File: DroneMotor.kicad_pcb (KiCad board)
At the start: 2 copper layers, 184 x 184 mm, 49 parts, among them Q1 ISCH54N04NM7V, Q10 ISCH54N04NM7V, Q11 ISCH54N04NM7V, Q12 ISCH54N04NM7V, Q13 ISCH54N04NM7V, Q14 ISCH54N04NM7V, Q15 ISCH54N04NM7V, Q16 ISCH54N04NM7V, Q17 ISCH54N04NM7V, Q18 ISCH54N04NM7V, Q19 ISCH54N04NM7V, Q2 ISCH54N04NM7V, Q20 ISCH54N04NM7V, Q21 ISCH54N04NM7V, Q22 ISCH54N04NM7V, Q23 ISCH54N04NM7V, Q24 ISCH54N04NM7V, Q3 ISCH54N04NM7V, Q4 ISCH54N04NM7V, Q5 ISCH54N04NM7V, Q6 ISCH54N04NM7V, Q7 ISCH54N04NM7V, Q8 ISCH54N04NM7V, Q9 ISCH54N04NM7V, U1 MKV58F1M0VLQ22, U10 UCC27211DRMR, U11 UCC27211DRMR, U12 UCC27211DRMR, U13 UCC27211DRMR, U2 UCC27211DRMR, U3 UCC27211DRMR, U4 UCC27211DRMR, U5 UCC27211DRMR, U6 UCC27211DRMR, U7 UCC27211DRMR, U8 UCC27211DRMR, U9 UCC27211DRMR

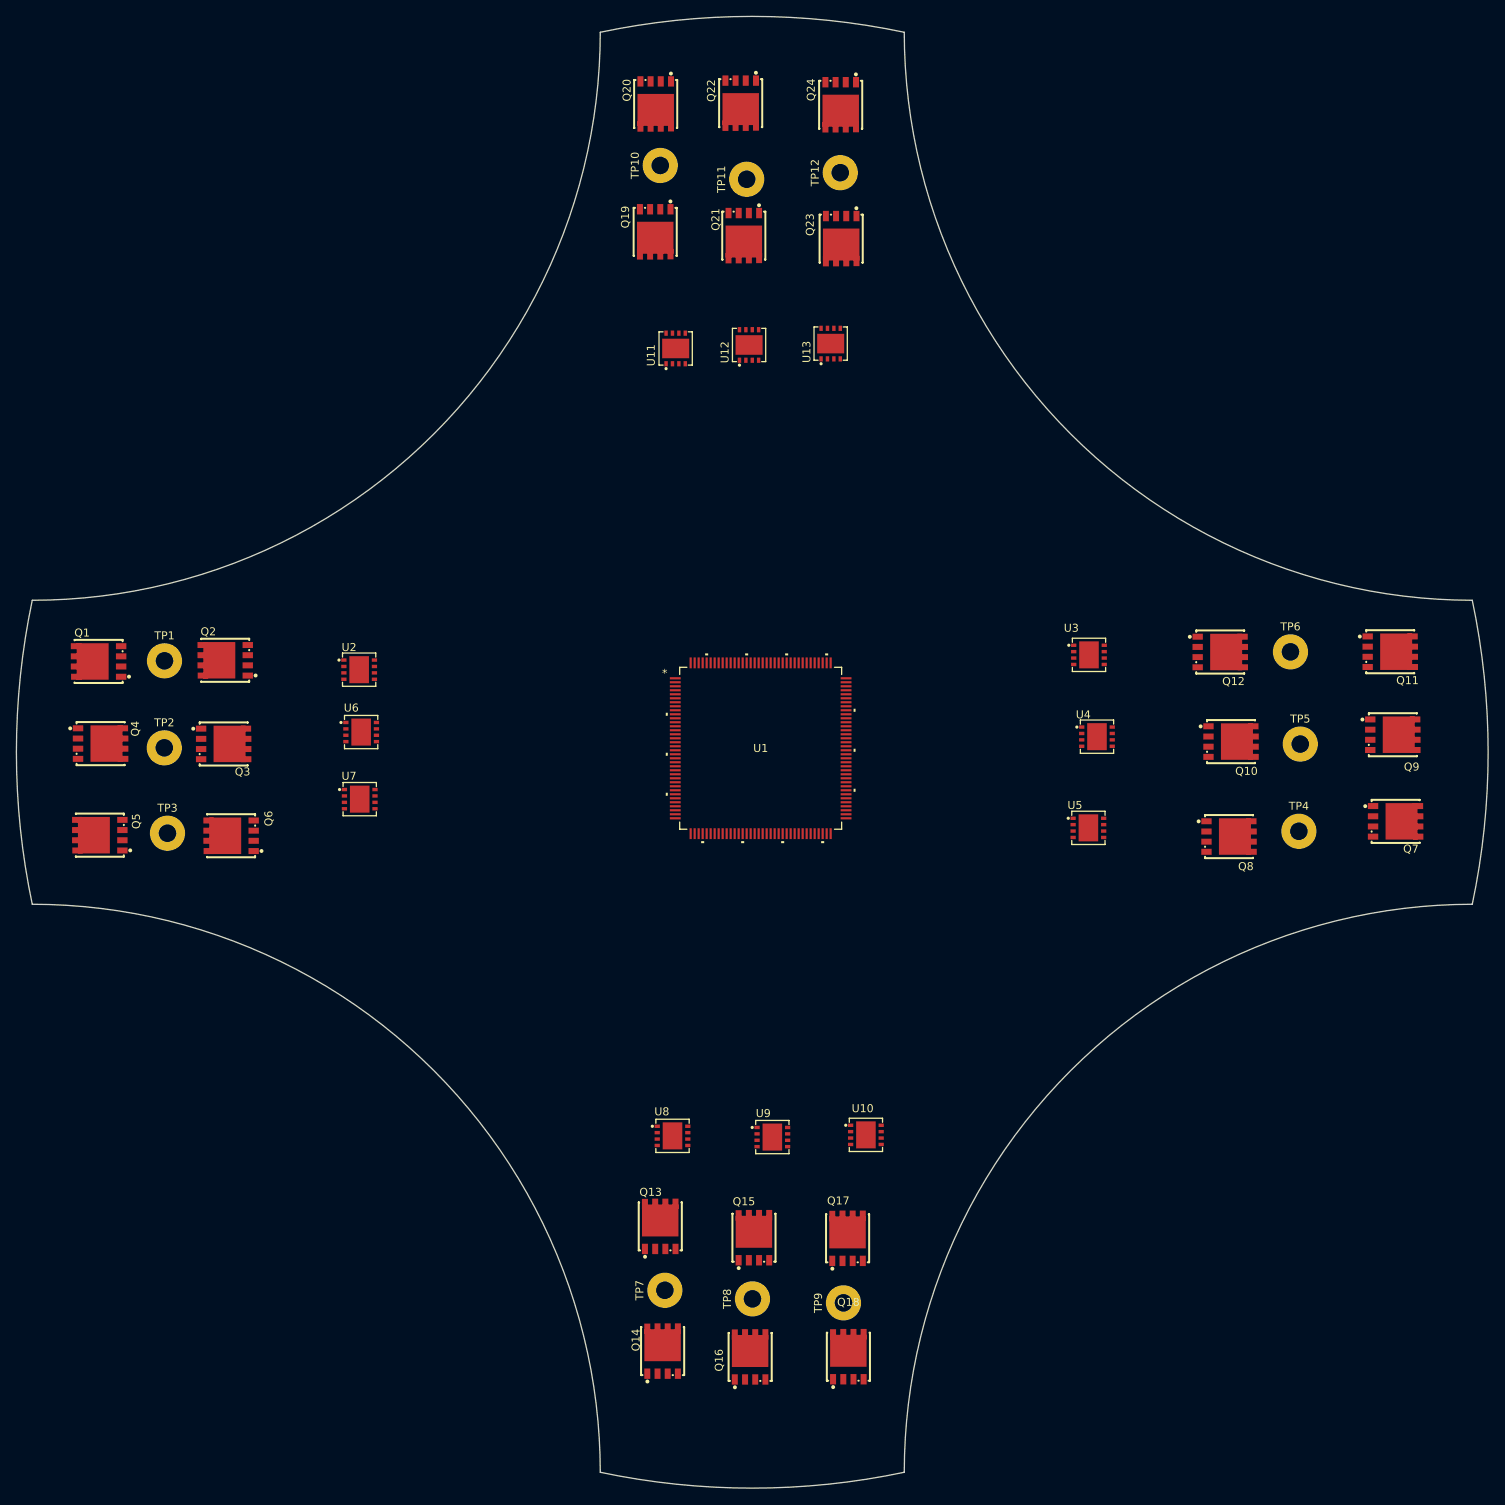
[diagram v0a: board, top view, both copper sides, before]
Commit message: add ti version
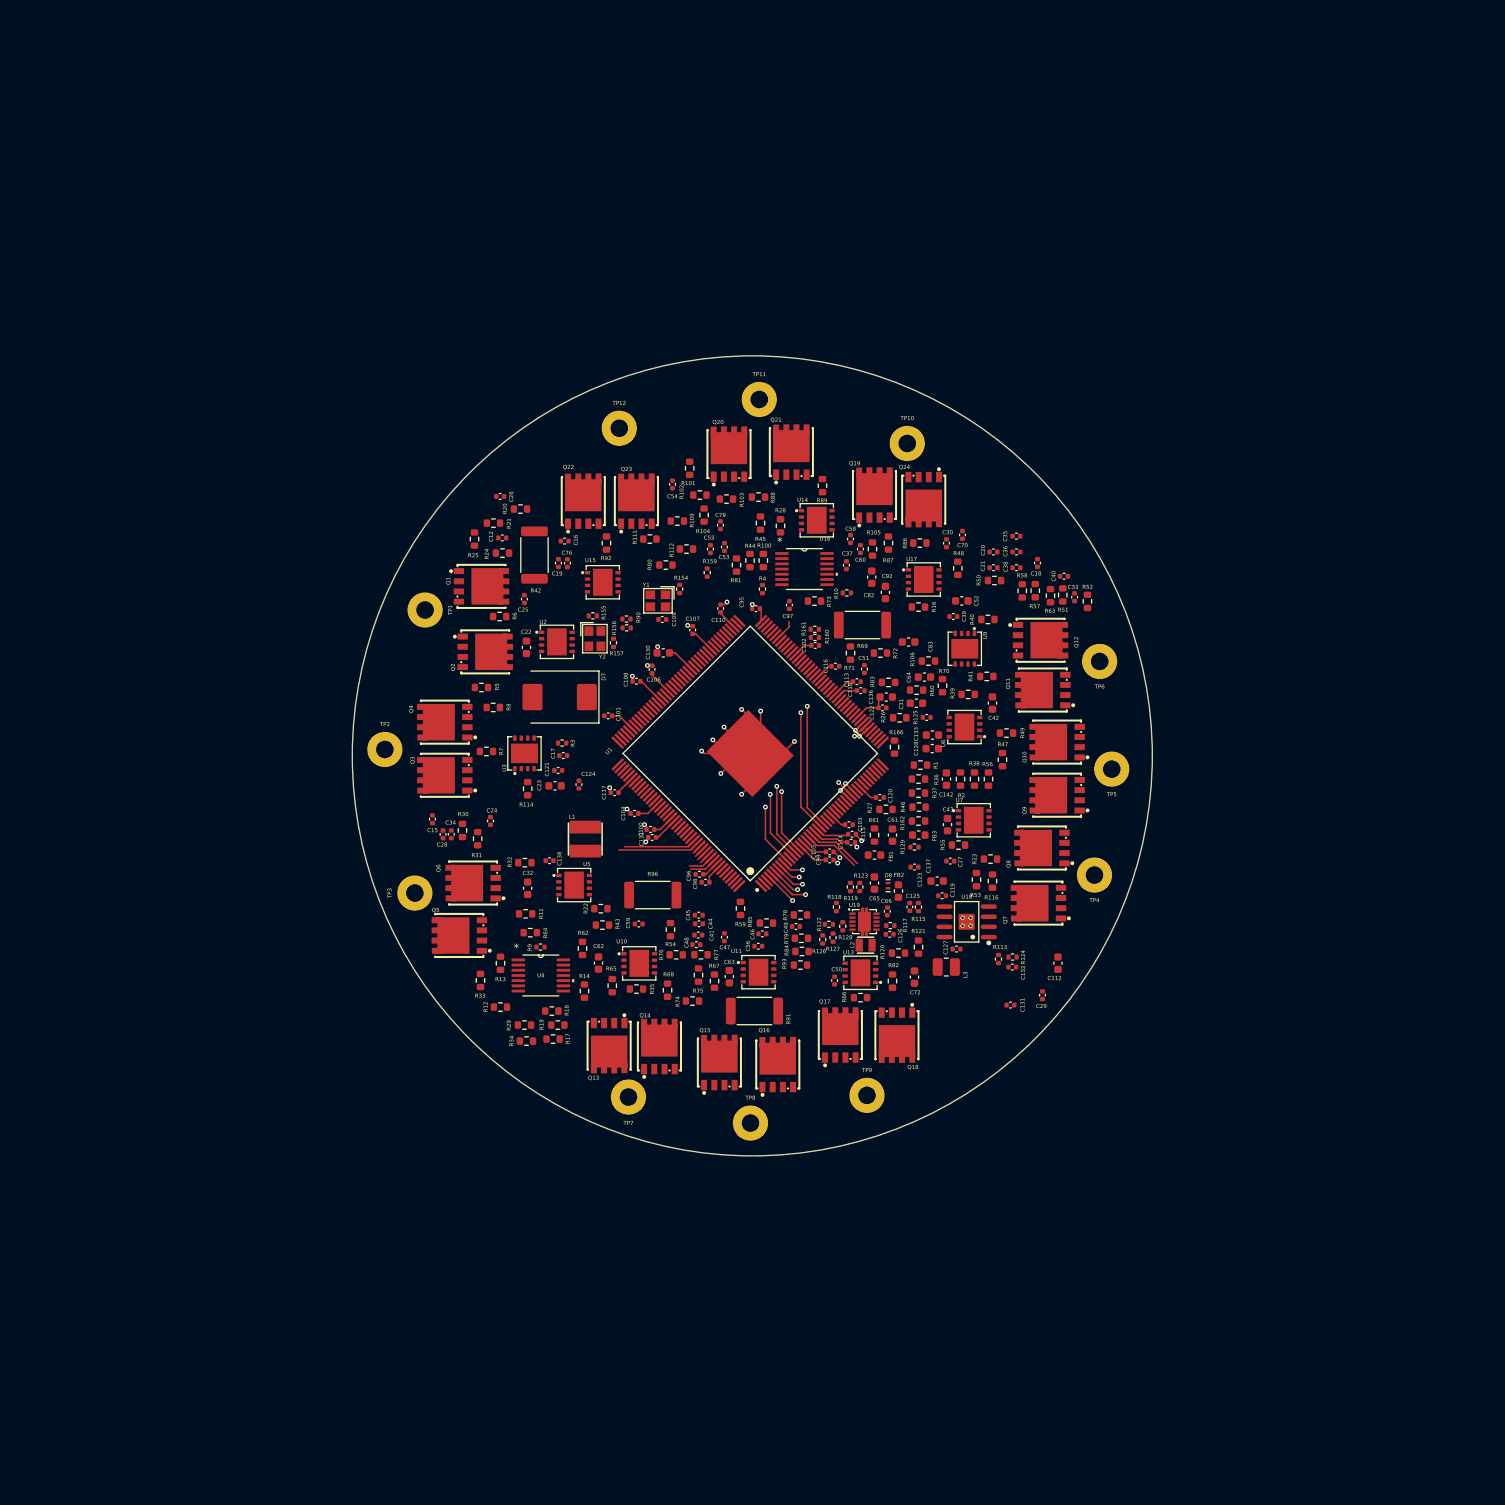
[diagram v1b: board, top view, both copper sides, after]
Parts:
- removed U12, U8: UCC27211DRMR, footprints:VSON-8_L4.0-W4.0-P0.80-TL-EP
- added C100: 0.1uF, Capacitor_SMD:C_0402_1005Metric, F.Cu at (202.0, 150.8)
- added C101: 0.1uF, Capacitor_SMD:C_0402_1005Metric, F.Cu at (196.7, 136.6)
- added C102: 0.1uF, Capacitor_SMD:C_0402_1005Metric, F.Cu at (222.6, 127.8)
- added C103: 0.1uF, Capacitor_SMD:C_0402_1005Metric, F.Cu at (226.8, 150.2)
- added C104: 0.1uF, Capacitor_SMD:C_0402_1005Metric, F.Cu at (200.0, 148.8)
- added C105: 0.1uF, Capacitor_SMD:C_0402_1005Metric, F.Cu at (224.4, 153.6)
- added C106: 0.1uF, Capacitor_SMD:C_0402_1005Metric, F.Cu at (202.2, 130.8)
- added C107: 0.1uF, Capacitor_SMD:C_0402_1005Metric, F.Cu at (207.3, 125.9)
- added C108: 0.1uF, Capacitor_SMD:C_0402_1005Metric, F.Cu at (200.2, 132.3)
- added C109: 0.1uF, Capacitor_SMD:C_0402_1005Metric, F.Cu at (203.5, 124.5)
- added C110: 0.1uF, Capacitor_SMD:C_0402_1005Metric, F.Cu at (210.8, 123.2)
- added C111: 0.1uF, Capacitor_SMD:C_0402_1005Metric, F.Cu at (202.2, 151.8)
- added C112: 3.3uF, Capacitor_SMD:C_0603_1608Metric, F.Cu at (252.9, 167.5)
- added C113: 0.1uF, Capacitor_SMD:C_0402_1005Metric, F.Cu at (227.8, 132.3)
- added C114: 0.1uF, Capacitor_SMD:C_0402_1005Metric, F.Cu at (227.1, 152.4)
- added C115: 0.1uF, Capacitor_SMD:C_0402_1005Metric, F.Cu at (227.2, 151.4)
- added C116: 0.1uF, Capacitor_SMD:C_0402_1005Metric, F.Cu at (225.1, 130.4)
- added C117: 0.1uF, Capacitor_SMD:C_0402_1005Metric, F.Cu at (197.5, 146.2)
- added C118: 0.1uF, Capacitor_SMD:C_0402_1005Metric, F.Cu at (228.3, 133.4)
- added C119: 0.1uF, Capacitor_SMD:C_0402_1005Metric, F.Cu at (238.5, 159.1)
- added C12: 2.2uF, Capacitor_SMD:C_0402_1005Metric, F.Cu at (183.5, 114.4)
- added C120: 0.1uF, Capacitor_SMD:C_0402_1005Metric, F.Cu at (230.7, 146.8)
- added C121: 1800pF, Capacitor_SMD:C_0402_1005Metric, F.Cu at (190.5, 143.4)
- added C122: 0.1uF, Capacitor_SMD:C_0402_1005Metric, F.Cu at (231.0, 135.6)
- added C123: 22uF, Capacitor_SMD:C_0603_1608Metric, F.Cu at (237.8, 157.2)
- added C124: 56pF, Capacitor_SMD:C_0402_1005Metric, F.Cu at (193.1, 145.2)
- added C125: 0.1uF, Capacitor_SMD:C_0402_1005Metric, F.Cu at (234.4, 160.5)
- added C126: 0.1uF, Capacitor_SMD:C_0402_1005Metric, F.Cu at (231.9, 163.9)
- added C127: 0.1uF, Capacitor_SMD:C_0402_1005Metric, F.Cu at (240.2, 165.8)
- added C128: 2.2uF, Capacitor_SMD:C_0603_1608Metric, F.Cu at (237.2, 140.7)
- added C130: 2.2uF, Capacitor_SMD:C_0603_1608Metric, F.Cu at (203.6, 128.7)
- added C131: 10uF, Capacitor_SMD:C_0402_1005Metric, F.Cu at (247.0, 172.8)
- added C132: 33pF, Capacitor_SMD:C_0402_1005Metric, F.Cu at (247.2, 168.0)
- added C133: 2.2uF, Capacitor_SMD:C_0603_1608Metric, F.Cu at (237.2, 139.0)
- added C136: 2.2uF, Capacitor_SMD:C_0603_1608Metric, F.Cu at (231.5, 134.2)
- added C137: 22uF, Capacitor_SMD:C_0402_1005Metric, F.Cu at (235.0, 155.5)
- added C138: 2.2uF, Capacitor_SMD:C_0402_1005Metric, F.Cu at (189.4, 154.7)
- added C142: 22uF, Capacitor_SMD:C_0603_1608Metric, F.Cu at (239.0, 144.5)
- added C15: 2.2uF, Capacitor_SMD:C_0402_1005Metric, F.Cu at (174.8, 149.5)
- added C16: 2.2uF, Capacitor_SMD:C_0402_1005Metric, F.Cu at (191.3, 114.8)
- added C17: 0.1uF, Capacitor_SMD:C_0402_1005Metric, F.Cu at (191.1, 141.6)
- added C18: 0.1uF, Capacitor_SMD:C_0402_1005Metric, F.Cu at (250.4, 117.5)
- added C19: 2.2uF, Capacitor_SMD:C_0402_1005Metric, F.Cu at (190.5, 117.5)
- added C20: 0.1uF, Capacitor_SMD:C_0402_1005Metric, F.Cu at (244.9, 116.1)
- added C21: 0.1uF, Capacitor_SMD:C_0402_1005Metric, F.Cu at (244.9, 118.1)
- added C22: 0.1uF, Capacitor_SMD:C_0603_1608Metric, F.Cu at (186.5, 128.0)
- added C23: 0.1uF, Capacitor_SMD:C_0603_1608Metric, F.Cu at (190.1, 145.3)
- added C24: 2.2uF, Capacitor_SMD:C_0402_1005Metric, F.Cu at (182.0, 149.7)
- added C25: 2.2uF, Capacitor_SMD:C_0402_1005Metric, F.Cu at (186.2, 122.0)
- added C26: 0.1uF, Capacitor_SMD:C_0402_1005Metric, F.Cu at (183.2, 109.2)
- added C27: 0.1uF, Capacitor_SMD:C_0402_1005Metric, F.Cu at (239.5, 154.8)
- added C28: 0.1uF, Capacitor_SMD:C_0402_1005Metric, F.Cu at (176.1, 151.4)
- added C29: 0.1uF, Capacitor_SMD:C_0402_1005Metric, F.Cu at (251.0, 171.5)
- added C30: 2.2uF, Capacitor_SMD:C_0402_1005Metric, F.Cu at (239.0, 115.0)
- added C31: 22uF, Capacitor_SMD:C_0603_1608Metric, F.Cu at (235.2, 135.0)
- added C32: 0.1uF, Capacitor_SMD:C_0603_1608Metric, F.Cu at (186.7, 158.2)
- added C33: 0.1uF, Capacitor_SMD:C_0402_1005Metric, F.Cu at (255.0, 121.8)
- added C34: 0.1uF, Capacitor_SMD:C_0402_1005Metric, F.Cu at (177.1, 151.4)
- added C35: 2.2uF, Capacitor_SMD:C_0402_1005Metric, F.Cu at (247.7, 114.1)
- added C36: 2.2uF, Capacitor_SMD:C_0402_1005Metric, F.Cu at (247.7, 116.1)
- added C37: 0.1uF, Capacitor_SMD:C_0402_1005Metric, F.Cu at (226.5, 117.8)
- added C38: 2.2uF, Capacitor_SMD:C_0402_1005Metric, F.Cu at (247.7, 118.1)
- added C39: 2.2uF, Capacitor_SMD:C_0402_1005Metric, F.Cu at (239.9, 124.2)
- added C40: 2.2uF, Capacitor_SMD:C_0402_1005Metric, F.Cu at (253.7, 119.2)
- added C41: 2.2uF, Capacitor_SMD:C_0402_1005Metric, F.Cu at (208.0, 164.0)
- added C42: 0.1uF, Capacitor_SMD:C_0603_1608Metric, F.Cu at (244.8, 135.0)
- added C43: 0.1uF, Capacitor_SMD:C_0603_1608Metric, F.Cu at (239.1, 150.2)
- added C44: 2.2uF, Capacitor_SMD:C_0402_1005Metric, F.Cu at (208.1, 162.6)
- added C45: 2.2uF, Capacitor_SMD:C_0402_1005Metric, F.Cu at (208.0, 161.5)
- added C46: 0.1uF, Capacitor_SMD:C_0402_1005Metric, F.Cu at (216.0, 163.8)
- added C47: 0.1uF, Capacitor_SMD:C_0402_1005Metric, F.Cu at (211.2, 164.3)
- added C48: 0.1uF, Capacitor_SMD:C_0402_1005Metric, F.Cu at (207.7, 165.2)
- added C49: 0.1uF, Capacitor_SMD:C_0402_1005Metric, F.Cu at (220.2, 162.9)
- added C50: 2.2uF, Capacitor_SMD:C_0402_1005Metric, F.Cu at (225.0, 169.7)
- added C51: 0.1uF, Capacitor_SMD:C_0402_1005Metric, F.Cu at (228.8, 130.8)
- added C52: 0.1uF, Capacitor_SMD:C_0603_1608Metric, F.Cu at (240.9, 122.2)
- added C53: 0.1uF, Capacitor_SMD:C_0402_1005Metric, F.Cu at (211.2, 115.5)
- added C54: 0.1uF, Capacitor_SMD:C_0402_1005Metric, F.Cu at (204.8, 107.7)
- added C55: 0.1uF, Capacitor_SMD:C_0402_1005Metric, F.Cu at (209.5, 115.8)
- added C56: 2.2uF, Capacitor_SMD:C_0402_1005Metric, F.Cu at (215.5, 165.4)
- added C58: 2.2uF, Capacitor_SMD:C_0402_1005Metric, F.Cu at (227.0, 114.5)
- added C59: 2.2uF, Capacitor_SMD:C_0402_1005Metric, F.Cu at (200.5, 162.6)
- added C60: 2.2uF, Capacitor_SMD:C_0402_1005Metric, F.Cu at (228.2, 115.8)
- added C61: 22uF, Capacitor_SMD:C_0603_1608Metric, F.Cu at (232.2, 151.5)
- added C62: 0.1uF, Capacitor_SMD:C_0603_1608Metric, F.Cu at (195.5, 167.5)
- added C63: 0.1uF, Capacitor_SMD:C_0603_1608Metric, F.Cu at (211.9, 169.2)
- added C64: 22uF, Capacitor_SMD:C_0603_1608Metric, F.Cu at (236.2, 131.8)
- added C65: 22uF, Capacitor_SMD:C_0603_1608Metric, F.Cu at (230.0, 157.5)
- added C66: 10uF, Capacitor_SMD:C_0402_1005Metric, F.Cu at (231.6, 161.0)
- added C70: 2.2uF, Capacitor_SMD:C_0402_1005Metric, F.Cu at (241.0, 114.0)
- added C72: 0.1uF, Capacitor_SMD:C_0603_1608Metric, F.Cu at (235.0, 169.2)
- added C76: 2.2uF, Capacitor_SMD:C_0402_1005Metric, F.Cu at (191.6, 117.5)
- added C79: 2.2uF, Capacitor_SMD:C_0402_1005Metric, F.Cu at (210.8, 112.8)
- added C82: 0.1uF, Capacitor_SMD:C_0603_1608Metric, F.Cu at (229.7, 119.3)
- added C83: 0.1uF, Capacitor_SMD:C_0603_1608Metric, F.Cu at (234.3, 127.4)
- added C92: 0.1uF, Capacitor_SMD:C_0603_1608Metric, F.Cu at (231.4, 121.2)
- added C95: 0.1uF, Capacitor_SMD:C_0402_1005Metric, F.Cu at (215.2, 123.2)
- added C96: 0.1uF, Capacitor_SMD:C_0402_1005Metric, F.Cu at (208.1, 156.4)
- added C97: 0.1uF, Capacitor_SMD:C_0402_1005Metric, F.Cu at (219.4, 122.7)
- added C98: 0.1uF, Capacitor_SMD:C_0402_1005Metric, F.Cu at (208.9, 157.4)
- added C99: 0.1uF, Capacitor_SMD:C_0402_1005Metric, F.Cu at (224.4, 154.6)
- added D7: SS510-SMC, Diode_SMD:D_SMC, F.Cu at (190.7, 134.2)
- added D8: CFSH05-20L, footprints:SOD-882_L1.0-W0.6-BI, F.Cu at (231.7, 157.8)
- added FB1: 60, Inductor_SMD:L_0603_1608Metric, F.Cu at (230.0, 154.0)
- added FB2: 220, Inductor_SMD:L_0603_1608Metric, F.Cu at (233.0, 158.5)
- added FB3: 60, Inductor_SMD:L_0603_1608Metric, F.Cu at (235.5, 151.5)
- added L1: 33uH, footprints:IND-SMD_L4.0-W4.0_FNR40XXS, F.Cu at (193.8, 152.0)
- added L2: VLS201612HBX-2R2M-1, footprints:IND-SMD_L2.0-W1.6_VLS201610ET, F.Cu at (228.9, 165.3)
- added L3: 3.3uH, Inductor_SMD:L_1008_2520Metric, F.Cu at (239.0, 168.0)
- added R1: 56.0, Resistor_SMD:R_0603_1608Metric, F.Cu at (235.8, 142.8)
- added R10: 330, Resistor_SMD:R_0402_1005Metric, F.Cu at (226.6, 121.2)
- added R100: 33K, Resistor_SMD:R_0603_1608Metric, F.Cu at (216.1, 117.2)
- added R101: 68K, Resistor_SMD:R_0603_1608Metric, F.Cu at (206.9, 105.7)
- added R102: 18K, Resistor_SMD:R_0603_1608Metric, F.Cu at (208.2, 109.0)
- added R103: 68K, Resistor_SMD:R_0603_1608Metric, F.Cu at (211.5, 109.5)
- added R104: 18K, Resistor_SMD:R_0603_1608Metric, F.Cu at (208.7, 111.5)
- added R105: 68K, Resistor_SMD:R_0603_1608Metric, F.Cu at (229.8, 115.8)
- added R106: 18K, Resistor_SMD:R_0603_1608Metric, F.Cu at (236.8, 129.8)
- added R109: 10, Resistor_SMD:R_0603_1608Metric, F.Cu at (205.4, 112.2)
- added R11: 10, Resistor_SMD:R_0603_1608Metric, F.Cu at (186.4, 161.3)
- added R111: 68K, Resistor_SMD:R_0603_1608Metric, F.Cu at (201.9, 114.5)
- added R112: 18K, Resistor_SMD:R_0603_1608Metric, F.Cu at (206.5, 115.8)
- added R113: 0, Resistor_SMD:R_0402_1005Metric, F.Cu at (245.5, 167.0)
- added R114: 32.4k, Resistor_SMD:R_0603_1608Metric, F.Cu at (186.7, 145.7)
- added R115: 22K, Resistor_SMD:R_0402_1005Metric, F.Cu at (235.5, 160.5)
- added R116: 178K, Resistor_SMD:R_0603_1608Metric, F.Cu at (244.8, 157.2)
- added R117: 0, Resistor_SMD:R_0402_1005Metric, F.Cu at (232.0, 162.8)
- added R118: 10K, Resistor_SMD:R_0402_1005Metric, F.Cu at (225.2, 160.5)
- added R119: 100K, Resistor_SMD:R_0402_1005Metric, F.Cu at (227.0, 158.0)
- added R12: 33K, Resistor_SMD:R_0603_1608Metric, F.Cu at (183.2, 173.0)
- added R120: 118K, Resistor_SMD:R_0603_1608Metric, F.Cu at (233.0, 166.2)
- added R121: 8.45K, Resistor_SMD:R_0603_1608Metric, F.Cu at (235.5, 165.5)
- added R122: 0, Resistor_SMD:R_0402_1005Metric, F.Cu at (224.3, 162.7)
- added R123: 56, Resistor_SMD:R_0402_1005Metric, F.Cu at (228.2, 158.0)
- added R124: 205K, Resistor_SMD:R_0402_1005Metric, F.Cu at (247.3, 166.8)
- added R125: 200K, Capacitor_SMD:C_0402_1005Metric, F.Cu at (236.5, 136.8)
- added R126: 340K, Resistor_SMD:R_0402_1005Metric, F.Cu at (223.5, 164.6)
- added R127: 2.00K, Resistor_SMD:R_0402_1005Metric, F.Cu at (224.8, 164.3)
- added R128: 75K, Resistor_SMD:R_0402_1005Metric, F.Cu at (226.0, 162.9)
- added R129: 680, Resistor_SMD:R_0402_1005Metric, F.Cu at (235.0, 153.0)
- added R13: 33K, Resistor_SMD:R_0603_1608Metric, F.Cu at (183.2, 167.5)
- added R14: 33K, Resistor_SMD:R_0603_1608Metric, F.Cu at (193.8, 171.0)
- added R154: 0, Resistor_SMD:R_0402_1005Metric, F.Cu at (205.7, 120.8)
- added R155: 0, Resistor_SMD:R_0402_1005Metric, F.Cu at (194.8, 124.1)
- added R156: 0, Resistor_SMD:R_0402_1005Metric, F.Cu at (199.0, 125.6)
- added R157: 0, Resistor_SMD:R_0402_1005Metric, F.Cu at (197.4, 127.5)
- added R159: 10K, Resistor_SMD:R_0402_1005Metric, F.Cu at (209.1, 118.7)
- added R16: 1K, Resistor_SMD:R_0603_1608Metric, F.Cu at (235.5, 123.0)
- added R160: 39, Resistor_SMD:R_0402_1005Metric, F.Cu at (222.6, 126.8)
- added R161: 2.2K, Resistor_SMD:R_0402_1005Metric, F.Cu at (222.5, 125.8)
- added R162: 0.1, Resistor_SMD:R_0603_1608Metric, F.Cu at (235.5, 149.8)
- added R166: 56.0, Resistor_SMD:R_0603_1608Metric, F.Cu at (232.5, 140.5)
- added R17: 1K, Resistor_SMD:R_0603_1608Metric, F.Cu at (189.8, 177.0)
- added R18: 33K, Resistor_SMD:R_0603_1608Metric, F.Cu at (189.7, 173.5)
- added R19: 33K, Resistor_SMD:R_0603_1608Metric, F.Cu at (190.4, 175.2)
- added R2: 56.0, Resistor_SMD:R_0603_1608Metric, F.Cu at (240.8, 144.5)
- added R20: 68K, Resistor_SMD:R_0603_1608Metric, F.Cu at (185.8, 110.8)
- added R21: 18K, Resistor_SMD:R_0603_1608Metric, F.Cu at (182.4, 112.5)
- added R22: 68K, Resistor_SMD:R_0603_1608Metric, F.Cu at (195.8, 160.7)
- added R23: 18K, Resistor_SMD:R_0603_1608Metric, F.Cu at (244.5, 154.5)
- added R24: 68K, Resistor_SMD:R_0603_1608Metric, F.Cu at (183.5, 116.2)
- added R25: 18K, Resistor_SMD:R_0603_1608Metric, F.Cu at (180.0, 114.5)
- added R26: 0.1, Resistor_SMD:R_0603_1608Metric, F.Cu at (233.2, 136.8)
- added R27: 0.1, Resistor_SMD:R_0603_1608Metric, F.Cu at (231.4, 148.3)
- added R28: 33K, Resistor_SMD:R_0603_1608Metric, F.Cu at (218.2, 112.8)
- added R29: 33K, Resistor_SMD:R_0603_1608Metric, F.Cu at (186.2, 175.2)
- added R3: 330, Resistor_SMD:R_0402_1005Metric, F.Cu at (191.0, 140.0)
- added R30: 68K, Resistor_SMD:R_0603_1608Metric, F.Cu at (178.5, 150.9)
- added R31: 18K, Resistor_SMD:R_0603_1608Metric, F.Cu at (180.4, 151.9)
- added R32: 10, Resistor_SMD:R_0603_1608Metric, F.Cu at (186.3, 154.9)
- added R33: 1K, Resistor_SMD:R_0603_1608Metric, F.Cu at (180.8, 169.7)
- added R34: 1K, Resistor_SMD:R_0603_1608Metric, F.Cu at (186.5, 177.2)
- added R35: 1K, Resistor_SMD:R_0603_1608Metric, F.Cu at (200.2, 170.8)
- added R36: 56.0, Resistor_SMD:R_0603_1608Metric, F.Cu at (235.5, 144.5)
- added R37: 56.0, Resistor_SMD:R_0603_1608Metric, F.Cu at (235.5, 146.2)
- added R38: 10, Resistor_SMD:R_0603_1608Metric, F.Cu at (242.5, 144.5)
- added R39: 10, Resistor_SMD:R_0603_1608Metric, F.Cu at (241.7, 133.9)
- added R4: 330, Resistor_SMD:R_0402_1005Metric, F.Cu at (216.0, 120.8)
- added R40: 10, Resistor_SMD:R_0603_1608Metric, F.Cu at (244.2, 124.5)
- added R41: 10, Resistor_SMD:R_0603_1608Metric, F.Cu at (244.0, 131.7)
- added R42: 0.002, Resistor_SMD:R_2512_6332Metric, F.Cu at (187.5, 116.5)
- added R43: 1K, Resistor_SMD:R_0603_1608Metric, F.Cu at (196.0, 162.8)
- added R44: 1K, Resistor_SMD:R_0603_1608Metric, F.Cu at (214.4, 117.2)
- added R45: 1K, Resistor_SMD:R_0603_1608Metric, F.Cu at (215.8, 112.5)
- added R46: 56.0, Resistor_SMD:R_0603_1608Metric, F.Cu at (235.6, 148.0)
- added R47: 68K, Resistor_SMD:R_0603_1608Metric, F.Cu at (246.0, 142.1)
- added R48: 18K, Resistor_SMD:R_0603_1608Metric, F.Cu at (240.4, 118.2)
- added R49: 68K, Resistor_SMD:R_0603_1608Metric, F.Cu at (246.5, 138.8)
- added R5: 10, Resistor_SMD:R_0603_1608Metric, F.Cu at (180.9, 133.1)
- added R50: 18K, Resistor_SMD:R_0603_1608Metric, F.Cu at (245.0, 119.7)
- added R51: 68K, Resistor_SMD:R_0603_1608Metric, F.Cu at (253.5, 121.5)
- added R52: 18K, Resistor_SMD:R_0603_1608Metric, F.Cu at (256.6, 122.3)
- added R53: 56.0, Resistor_SMD:R_0603_1608Metric, F.Cu at (242.8, 157.1)
- added R54: 56.0, Resistor_SMD:R_0603_1608Metric, F.Cu at (204.5, 163.3)
- added R55: 10, Resistor_SMD:R_0603_1608Metric, F.Cu at (240.5, 152.8)
- added R56: 10, Resistor_SMD:R_0603_1608Metric, F.Cu at (244.2, 144.5)
- added R57: 68K, Resistor_SMD:R_0603_1608Metric, F.Cu at (250.1, 121.0)
- added R58: 18K, Resistor_SMD:R_0603_1608Metric, F.Cu at (248.5, 121.0)
- added R59: 56.0, Resistor_SMD:R_0603_1608Metric, F.Cu at (213.2, 160.7)
- added R6: 10, Resistor_SMD:R_0603_1608Metric, F.Cu at (183.1, 124.2)
- added R60: 56.0, Resistor_SMD:R_0603_1608Metric, F.Cu at (235.3, 133.4)
- added R61: 56.0, Resistor_SMD:R_0603_1608Metric, F.Cu at (230.0, 151.5)
- added R62: 56.0, Resistor_SMD:R_0603_1608Metric, F.Cu at (193.5, 165.7)
- added R63: 56.0, Resistor_SMD:R_0603_1608Metric, F.Cu at (252.0, 121.6)
- added R64: 56.0, Resistor_SMD:R_0603_1608Metric, F.Cu at (187.0, 163.7)
- added R65: 10, Resistor_SMD:R_0603_1608Metric, F.Cu at (197.2, 170.3)
- added R66: 10, Resistor_SMD:R_0603_1608Metric, F.Cu at (228.2, 171.8)
- added R67: 10, Resistor_SMD:R_0603_1608Metric, F.Cu at (210.0, 169.8)
- added R68: 10, Resistor_SMD:R_0603_1608Metric, F.Cu at (204.1, 170.9)
- added R69: 0.002, Resistor_SMD:R_2512_6332Metric, F.Cu at (228.5, 125.2)
- added R7: 10, Resistor_SMD:R_0603_1608Metric, F.Cu at (181.5, 141.1)
- added R70: 56.0, Resistor_SMD:R_0603_1608Metric, F.Cu at (238.5, 132.8)
- added R71: 56.0, Resistor_SMD:R_0603_1608Metric, F.Cu at (227.0, 128.8)
- added R72: 56.0, Resistor_SMD:R_0603_1608Metric, F.Cu at (230.8, 128.8)
- added R73: 56.0, Resistor_SMD:R_0603_1608Metric, F.Cu at (222.5, 122.2)
- added R74: 68K, Resistor_SMD:R_0603_1608Metric, F.Cu at (207.2, 172.2)
- added R75: 18K, Resistor_SMD:R_0603_1608Metric, F.Cu at (208.0, 169.0)
- added R76: 68K, Resistor_SMD:R_0603_1608Metric, F.Cu at (205.2, 166.5)
- added R77: 18K, Resistor_SMD:R_0603_1608Metric, F.Cu at (208.3, 166.5)
- added R78: 68K, Resistor_SMD:R_0603_1608Metric, F.Cu at (220.8, 161.5)
- added R79: 18K, Resistor_SMD:R_0603_1608Metric, F.Cu at (220.9, 164.4)
- added R8: 10, Resistor_SMD:R_0603_1608Metric, F.Cu at (182.3, 135.6)
- added R80: 56.0, Resistor_SMD:R_0603_1608Metric, F.Cu at (203.9, 117.8)
- added R81: 56.0, Resistor_SMD:R_0603_1608Metric, F.Cu at (212.8, 117.8)
- added R82: 10, Resistor_SMD:R_0603_1608Metric, F.Cu at (232.2, 169.8)
- added R83: 0.1, Resistor_SMD:R_0603_1608Metric, F.Cu at (231.8, 132.4)
- added R84: 68K, Resistor_SMD:R_0603_1608Metric, F.Cu at (220.9, 166.1)
- added R85: 18K, Resistor_SMD:R_0603_1608Metric, F.Cu at (216.5, 162.5)
- added R86: 10, Resistor_SMD:R_0603_1608Metric, F.Cu at (235.7, 115.0)
- added R87: 10, Resistor_SMD:R_0603_1608Metric, F.Cu at (231.8, 115.0)
- added R88: 10, Resistor_SMD:R_0603_1608Metric, F.Cu at (215.5, 109.2)
- added R89: 10, Resistor_SMD:R_0603_1608Metric, F.Cu at (223.5, 107.8)
- added R9: 330, Resistor_SMD:R_0402_1005Metric, F.Cu at (188.2, 165.5)
- added R90: 2.2K, Resistor_SMD:R_0402_1005Metric, F.Cu at (199.0, 124.5)
- added R91: 0.002, Resistor_SMD:R_2512_6332Metric, F.Cu at (215.0, 173.5)
- added R92: 10, Resistor_SMD:R_0603_1608Metric, F.Cu at (196.5, 115.0)
- added R93: 10, Resistor_SMD:R_0603_1608Metric, F.Cu at (220.8, 167.8)
- added R96: 0.002, Resistor_SMD:R_2512_6332Metric, F.Cu at (202.3, 159.0)
- added U14: UCC27211DRMR, footprints:VSON-8_L4.0-W4.0-P0.80-TL-EP, F.Cu at (222.8, 112.2)
- added U15: UCC27211DRMR, footprints:VSON-8_L4.0-W4.0-P0.80-TL-EP, F.Cu at (196.0, 119.9)
- added U16: OPA4374AIPWR, footprints:PW14, F.Cu at (221.2, 118.2)
- added U17: UCC27211DRMR, footprints:VSON-8_L4.0-W4.0-P0.80-TL-EP, F.Cu at (236.2, 119.5)
- added U18: TPS54360DDAR, footprints:SOIC-8_L5.0-W4.0-P1.27-LS6.0-BL-EP2.0, F.Cu at (241.5, 162.3)
- added U19: TPS62420DRCR, footprints:VSON-10_L3.0-W3.0-P0.50-TL-EP, F.Cu at (228.8, 162.3)
- added Y1: OT3EL89CJI-111YLC-25M, footprints:OSC-SMD_4P-L2.5-W2.0-BL, F.Cu at (202.9, 122.2)
- added Y2: OT3EL89CJI-111YLC-20M, footprints:OSC-SMD_4P-L2.5-W2.0-BL, F.Cu at (195.1, 127.0)
- U1: value MKV58F1M0VLQ22 -> XF28388DPTPS; footprint footprints:LQFP144_SOT486-2_NXP -> footprints:PTP0176F-IPC_A
- U4: value UCC27211DRMR -> OPA4374AIPWR; footprint footprints:VSON-8_L4.0-W4.0-P0.80-TL-EP -> footprints:PW14
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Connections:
- net /Controller/M1_BEMF_C renamed /Controller/EPWM14A
- net /Controller/M2_BEMF_C renamed /controllerConfig/MCU_TCK
- net /Controller/M2_PWM_B_LS renamed /controllerConfig/MCU_XRSn
- net /Controller/M3_BEMF_A renamed /Controller/EPWM14B
- net /Controller/M3_DRV_OC renamed /Controller/EPWM15A
- net /Controller/M4_DRV_OC renamed /Controller/EPWM15B
- net /Controller/MOSI renamed I2CA_SCL
- net /Controller/SCLK renamed I2CA_SDA
- net /Controller/UART_TX renamed /Controller/EPWM13B
- net /Controller/U_DCB renamed /Controller/EPWM13A
- net Net-(Q19-S-Pad1) renamed /motor4/PA_HS_S
- net Net-(Q21-S-Pad1) renamed /motor4/PB_HS_S
- net Net-(Q23-S-Pad1) renamed /motor4/PC_HS_S
- Q1 pad 1: Net-(Q1-S-Pad1) -> /motor1/PA_HS_S
- Q1 pad 2: Net-(Q1-S-Pad1) -> /motor1/PA_HS_S
- Q1 pad 3: Net-(Q1-S-Pad1) -> /motor1/PA_HS_S
- Q1 pad 5: Net-(Q1-D-Pad5) -> VCC_DC+
- Q1 pad 6: Net-(Q1-D-Pad5) -> VCC_DC+
- Q1 pad 7: Net-(Q1-D-Pad5) -> VCC_DC+
- Q1 pad 8: Net-(Q1-D-Pad5) -> VCC_DC+
- Q10 pad 5: Net-(Q10-D-Pad5) -> /motor2/PB_HS_S
- Q10 pad 6: Net-(Q10-D-Pad5) -> /motor2/PB_HS_S
- Q10 pad 7: Net-(Q10-D-Pad5) -> /motor2/PB_HS_S
- Q10 pad 8: Net-(Q10-D-Pad5) -> /motor2/PB_HS_S
- Q11 pad 1: Net-(Q11-S-Pad1) -> /motor2/PC_HS_S
- Q11 pad 2: Net-(Q11-S-Pad1) -> /motor2/PC_HS_S
- Q11 pad 3: Net-(Q11-S-Pad1) -> /motor2/PC_HS_S
- Q11 pad 5: Net-(Q11-D-Pad5) -> VCC_DC+
- Q11 pad 6: Net-(Q11-D-Pad5) -> VCC_DC+
- Q11 pad 7: Net-(Q11-D-Pad5) -> VCC_DC+
- Q11 pad 8: Net-(Q11-D-Pad5) -> VCC_DC+
- Q12 pad 1: Net-(Q12-S-Pad1) -> Net-(Q10-S-Pad1)
- Q12 pad 2: Net-(Q12-S-Pad1) -> Net-(Q10-S-Pad1)
- Q12 pad 3: Net-(Q12-S-Pad1) -> Net-(Q10-S-Pad1)
- Q12 pad 5: Net-(Q11-S-Pad1) -> /motor2/PC_HS_S
- Q12 pad 6: Net-(Q11-S-Pad1) -> /motor2/PC_HS_S
- Q12 pad 7: Net-(Q11-S-Pad1) -> /motor2/PC_HS_S
- Q12 pad 8: Net-(Q11-S-Pad1) -> /motor2/PC_HS_S
- Q13 pad 1: Net-(Q13-S-Pad1) -> /motor3/PA_HS_S
- Q13 pad 2: Net-(Q13-S-Pad1) -> /motor3/PA_HS_S
- Q13 pad 3: Net-(Q13-S-Pad1) -> /motor3/PA_HS_S
- Q13 pad 5: Net-(Q13-D-Pad5) -> VCC_DC+
- Q13 pad 6: Net-(Q13-D-Pad5) -> VCC_DC+
- Q13 pad 7: Net-(Q13-D-Pad5) -> VCC_DC+
- Q13 pad 8: Net-(Q13-D-Pad5) -> VCC_DC+
- Q14 pad 5: Net-(Q13-S-Pad1) -> /motor3/PA_HS_S
- Q14 pad 6: Net-(Q13-S-Pad1) -> /motor3/PA_HS_S
- Q14 pad 7: Net-(Q13-S-Pad1) -> /motor3/PA_HS_S
- Q14 pad 8: Net-(Q13-S-Pad1) -> /motor3/PA_HS_S
- Q15 pad 1: Net-(Q15-S-Pad1) -> /motor3/PB_HS_S
- Q15 pad 2: Net-(Q15-S-Pad1) -> /motor3/PB_HS_S
- Q15 pad 3: Net-(Q15-S-Pad1) -> /motor3/PB_HS_S
- Q15 pad 5: Net-(Q13-D-Pad5) -> VCC_DC+
- Q15 pad 6: Net-(Q13-D-Pad5) -> VCC_DC+
- Q15 pad 7: Net-(Q13-D-Pad5) -> VCC_DC+
- Q15 pad 8: Net-(Q13-D-Pad5) -> VCC_DC+
- Q16 pad 1: Net-(Q16-S-Pad1) -> Net-(Q14-S-Pad1)
- Q16 pad 2: Net-(Q16-S-Pad1) -> Net-(Q14-S-Pad1)
- Q16 pad 3: Net-(Q16-S-Pad1) -> Net-(Q14-S-Pad1)
- Q16 pad 5: Net-(Q15-S-Pad1) -> /motor3/PB_HS_S
- Q16 pad 6: Net-(Q15-S-Pad1) -> /motor3/PB_HS_S
- Q16 pad 7: Net-(Q15-S-Pad1) -> /motor3/PB_HS_S
- Q16 pad 8: Net-(Q15-S-Pad1) -> /motor3/PB_HS_S
- Q17 pad 1: Net-(Q17-S-Pad1) -> /motor3/PC_HS_S
- Q17 pad 2: Net-(Q17-S-Pad1) -> /motor3/PC_HS_S
- Q17 pad 3: Net-(Q17-S-Pad1) -> /motor3/PC_HS_S
- Q17 pad 5: Net-(Q13-D-Pad5) -> VCC_DC+
- Q17 pad 6: Net-(Q13-D-Pad5) -> VCC_DC+
- Q17 pad 7: Net-(Q13-D-Pad5) -> VCC_DC+
- Q17 pad 8: Net-(Q13-D-Pad5) -> VCC_DC+
- Q18 pad 1: Net-(Q18-S-Pad1) -> Net-(Q14-S-Pad1)
- Q18 pad 2: Net-(Q18-S-Pad1) -> Net-(Q14-S-Pad1)
- Q18 pad 3: Net-(Q18-S-Pad1) -> Net-(Q14-S-Pad1)
- Q18 pad 5: Net-(Q17-S-Pad1) -> /motor3/PC_HS_S
- Q18 pad 6: Net-(Q17-S-Pad1) -> /motor3/PC_HS_S
- Q18 pad 7: Net-(Q17-S-Pad1) -> /motor3/PC_HS_S
- Q18 pad 8: Net-(Q17-S-Pad1) -> /motor3/PC_HS_S
- Q19 pad 5: Net-(Q19-D-Pad5) -> VCC_DC+
- Q19 pad 6: Net-(Q19-D-Pad5) -> VCC_DC+
- Q19 pad 7: Net-(Q19-D-Pad5) -> VCC_DC+
- Q19 pad 8: Net-(Q19-D-Pad5) -> VCC_DC+
- Q2 pad 5: Net-(Q1-S-Pad1) -> /motor1/PA_HS_S
- Q2 pad 6: Net-(Q1-S-Pad1) -> /motor1/PA_HS_S
- Q2 pad 7: Net-(Q1-S-Pad1) -> /motor1/PA_HS_S
- Q2 pad 8: Net-(Q1-S-Pad1) -> /motor1/PA_HS_S
- Q20 pad 1: Net-(Q20-S-Pad1) -> GNDREF
- Q20 pad 2: Net-(Q20-S-Pad1) -> GNDREF
- Q20 pad 3: Net-(Q20-S-Pad1) -> GNDREF
- Q21 pad 5: Net-(Q19-D-Pad5) -> VCC_DC+
- Q21 pad 6: Net-(Q19-D-Pad5) -> VCC_DC+
- Q21 pad 7: Net-(Q19-D-Pad5) -> VCC_DC+
- Q21 pad 8: Net-(Q19-D-Pad5) -> VCC_DC+
- Q22 pad 1: Net-(Q22-S-Pad1) -> GNDREF
- Q22 pad 2: Net-(Q22-S-Pad1) -> GNDREF
- Q22 pad 3: Net-(Q22-S-Pad1) -> GNDREF
- Q23 pad 5: Net-(Q19-D-Pad5) -> VCC_DC+
- Q23 pad 6: Net-(Q19-D-Pad5) -> VCC_DC+
- Q23 pad 7: Net-(Q19-D-Pad5) -> VCC_DC+
- Q23 pad 8: Net-(Q19-D-Pad5) -> VCC_DC+
- Q24 pad 1: Net-(Q24-S-Pad1) -> GNDREF
- Q24 pad 2: Net-(Q24-S-Pad1) -> GNDREF
- Q24 pad 3: Net-(Q24-S-Pad1) -> GNDREF
- Q3 pad 1: Net-(Q3-S-Pad1) -> /motor1/PB_HS_S
- Q3 pad 2: Net-(Q3-S-Pad1) -> /motor1/PB_HS_S
- Q3 pad 3: Net-(Q3-S-Pad1) -> /motor1/PB_HS_S
- Q3 pad 5: Net-(Q1-D-Pad5) -> VCC_DC+
- Q3 pad 6: Net-(Q1-D-Pad5) -> VCC_DC+
- Q3 pad 7: Net-(Q1-D-Pad5) -> VCC_DC+
- Q3 pad 8: Net-(Q1-D-Pad5) -> VCC_DC+
- Q4 pad 1: Net-(Q4-S-Pad1) -> Net-(Q2-S-Pad1)
- Q4 pad 2: Net-(Q4-S-Pad1) -> Net-(Q2-S-Pad1)
- Q4 pad 3: Net-(Q4-S-Pad1) -> Net-(Q2-S-Pad1)
- Q4 pad 5: Net-(Q3-S-Pad1) -> /motor1/PB_HS_S
- Q4 pad 6: Net-(Q3-S-Pad1) -> /motor1/PB_HS_S
- Q4 pad 7: Net-(Q3-S-Pad1) -> /motor1/PB_HS_S
- Q4 pad 8: Net-(Q3-S-Pad1) -> /motor1/PB_HS_S
- Q5 pad 1: Net-(Q5-S-Pad1) -> /motor1/PC_HS_S
- Q5 pad 2: Net-(Q5-S-Pad1) -> /motor1/PC_HS_S
- Q5 pad 3: Net-(Q5-S-Pad1) -> /motor1/PC_HS_S
- Q5 pad 5: Net-(Q1-D-Pad5) -> VCC_DC+
- Q5 pad 6: Net-(Q1-D-Pad5) -> VCC_DC+
- Q5 pad 7: Net-(Q1-D-Pad5) -> VCC_DC+
- Q5 pad 8: Net-(Q1-D-Pad5) -> VCC_DC+
- Q6 pad 1: Net-(Q6-S-Pad1) -> Net-(Q2-S-Pad1)
- Q6 pad 2: Net-(Q6-S-Pad1) -> Net-(Q2-S-Pad1)
- Q6 pad 3: Net-(Q6-S-Pad1) -> Net-(Q2-S-Pad1)
- Q6 pad 5: Net-(Q5-S-Pad1) -> /motor1/PC_HS_S
- Q6 pad 6: Net-(Q5-S-Pad1) -> /motor1/PC_HS_S
- Q6 pad 7: Net-(Q5-S-Pad1) -> /motor1/PC_HS_S
- Q6 pad 8: Net-(Q5-S-Pad1) -> /motor1/PC_HS_S
- Q7 pad 1: Net-(Q7-S-Pad1) -> /motor2/PA_HS_S
- Q7 pad 2: Net-(Q7-S-Pad1) -> /motor2/PA_HS_S
- Q7 pad 3: Net-(Q7-S-Pad1) -> /motor2/PA_HS_S
- Q7 pad 5: Net-(Q11-D-Pad5) -> VCC_DC+
- Q7 pad 6: Net-(Q11-D-Pad5) -> VCC_DC+
- Q7 pad 7: Net-(Q11-D-Pad5) -> VCC_DC+
- Q7 pad 8: Net-(Q11-D-Pad5) -> VCC_DC+
- Q8 pad 1: Net-(Q8-S-Pad1) -> Net-(Q10-S-Pad1)
- Q8 pad 2: Net-(Q8-S-Pad1) -> Net-(Q10-S-Pad1)
- Q8 pad 3: Net-(Q8-S-Pad1) -> Net-(Q10-S-Pad1)
- Q8 pad 5: Net-(Q7-S-Pad1) -> /motor2/PA_HS_S
- Q8 pad 6: Net-(Q7-S-Pad1) -> /motor2/PA_HS_S
- Q8 pad 7: Net-(Q7-S-Pad1) -> /motor2/PA_HS_S
- Q8 pad 8: Net-(Q7-S-Pad1) -> /motor2/PA_HS_S
- Q9 pad 1: Net-(Q10-D-Pad5) -> /motor2/PB_HS_S
- Q9 pad 2: Net-(Q10-D-Pad5) -> /motor2/PB_HS_S
- Q9 pad 3: Net-(Q10-D-Pad5) -> /motor2/PB_HS_S
- Q9 pad 5: Net-(Q11-D-Pad5) -> VCC_DC+
- Q9 pad 6: Net-(Q11-D-Pad5) -> VCC_DC+
- Q9 pad 7: Net-(Q11-D-Pad5) -> VCC_DC+
- Q9 pad 8: Net-(Q11-D-Pad5) -> VCC_DC+
- TP1 pad 1: Net-(Q1-S-Pad1) -> /motor1/PA_HS_S
- TP2 pad 1: Net-(Q3-S-Pad1) -> /motor1/PB_HS_S
- TP3 pad 1: Net-(Q5-S-Pad1) -> /motor1/PC_HS_S
- TP4 pad 1: Net-(Q7-S-Pad1) -> /motor2/PA_HS_S
- TP5 pad 1: Net-(Q10-D-Pad5) -> /motor2/PB_HS_S
- TP6 pad 1: Net-(Q11-S-Pad1) -> /motor2/PC_HS_S
- TP7 pad 1: Net-(Q13-S-Pad1) -> /motor3/PA_HS_S
- TP8 pad 1: Net-(Q15-S-Pad1) -> /motor3/PB_HS_S
- TP9 pad 1: Net-(Q17-S-Pad1) -> /motor3/PC_HS_S
- U1 pad 1: /Controller/M1_DRV_INT -> /Controller/EPWM6A
- U1 pad 10: unconnected-(U1-FTM3_CH2-Pad10) -> /Controller/EPWM10A
- U1 pad 100: /Controller/M2_INPUT -> unconnected-(U1D-GPIO55-Pad100)
- U1 pad 101: /Controller/M3_INPUT -> unconnected-(U1D-GPIO56-Pad101)
- U1 pad 102: /Controller/M4_INPUT -> unconnected-(U1D-GPIO57-Pad102)
- U1 pad 103: /Controller/M1_SS -> unconnected-(U1D-GPIO58-Pad103)
- U1 pad 104: /Controller/M2_SS -> unconnected-(U1D-GPIO59-Pad104)
- U1 pad 105: /Controller/M3_SS -> unconnected-(U1D-GPIO60-Pad105)
- U1 pad 106: /Controller/M4_SS -> VDD_3V3
- U1 pad 107: GNDD -> unconnected-(U1D-GPIO61-Pad107)
- U1 pad 108: +3.3V -> unconnected-(U1D-GPIO62-Pad108)
- U1 pad 109: /Controller/M4_DRV_INT -> unconnected-(U1D-GPIO63-Pad109)
- U1 pad 11: unconnected-(U1-FTM3_CH3-Pad11) -> VDD_3V3
- U1 pad 110: /Controller/M4_PWM_A_LS -> unconnected-(U1D-GPIO64-Pad110)
- U1 pad 111: /Controller/M4_PWM_B_LS -> unconnected-(U1D-GPIO65-Pad111)
- U1 pad 112: /Controller/M4_PWM_C_LS -> unconnected-(U1D-GPIO66-Pad112)
- U1 pad 113: /Controller/M3_PWM_C_HS -> unconnected-(U1C-GPIO44-Pad113)
- U1 pad 114: /Controller/M4_PWM_C_HS -> VDD_3V3
- U1 pad 115: /Controller/M1_INPUT -> unconnected-(U1C-GPIO45-Pad115)
- U1 pad 116: /Controller/M2_INPUT -> VDD_3V3
- U1 pad 117: /Controller/M1_PWM_A_HS -> VDD_1V2
- U1 pad 118: /Controller/M1_PWM_B_LS -> unconnected-(U1D-GPIO133-Pad118)
- U1 pad 119: /Controller/M1_PWM_C_LS -> unconnected-(U1A-NC-Pad119)
- U1 pad 12: unconnected-(U1-FTM3_CH4-Pad12) -> /Controller/EPWM10B
- U1 pad 120: /Controller/DRV_EN -> GNDD
- U1 pad 121: GNDD -> unconnected-(U1A-X2-Pad121)
- U1 pad 122: +3.3V -> GNDD
- U1 pad 123: /Controller/M2_PWM_A_LS -> /controllerConfig/F2838x_CLK
- U1 pad 125: /Controller/M2_PWM_C_LS -> GNDD
- U1 pad 126: unconnected-(U1-FB_TA-Pad126) -> VDD_1V2
- U1 pad 127: /Controller/M1_PWM_A_HS -> VDD_3V3
- U1 pad 128: /Controller/M2_PWM_A_HS -> unconnected-(U1C-GPIO46-Pad128)
- U1 pad 129: /Controller/M1_PWM_B_HS -> unconnected-(U1C-GPIO47-Pad129)
- U1 pad 13: unconnected-(U1-FTM3_CH5-Pad13) -> /Controller/EPWM11A
- U1 pad 130: /Controller/M2_PWM_B_HS -> unconnected-(U1C-GPIO42-Pad130)
- U1 pad 131: /Controller/M1_PWM_C_HS -> unconnected-(U1C-GPIO43-Pad131)
- U1 pad 132: /Controller/M2_PWM_C_HS -> unconnected-(U1D-GPIO67-Pad132)
- U1 pad 133: /Controller/M3_INPUT -> unconnected-(U1D-GPIO68-Pad133)
- U1 pad 134: GNDD -> unconnected-(U1D-GPIO69-Pad134)
- U1 pad 135: +3.3V -> unconnected-(U1D-GPIO70-Pad135)
- U1 pad 136: /Controller/M4_INPUT -> unconnected-(U1D-GPIO71-Pad136)
- U1 pad 137: unconnected-(U1-FB_A16-Pad137) -> VDD_1V2
- U1 pad 138: unconnected-(U1-FB_A17-Pad138) -> VDD_3V3
- U1 pad 14: unconnected-(U1-FTM3_CH6-Pad14) -> /Controller/EPWM11B
- U1 pad 15: unconnected-(U1-FTM3_CH7-Pad15) -> VDD_3V3
- U1 pad 16: +3.3V -> VDD_1V2
- U1 pad 17: GNDD -> unconnected-(U1D-GPIO99-Pad17)
- U1 pad 18: /Controller/M1_BEMF_A -> /Controller/EPWM5A
- U1 pad 19: /Controller/M1_BEMF_B -> /Controller/EPWM5B
- U1 pad 2: /Controller/M2_DRV_INT -> /Controller/EPWM6B
- U1 pad 20: /Controller/M2_BEMF_A -> VDD_3V3
- U1 pad 21: /Controller/M2_BEMF_B -> VDD_1V2
- U1 pad 22: GNDD -> /Controller/EPWM12A
- U1 pad 23: /Controller/M1_I_DCB -> /Controller/EPWM12B
- U1 pad 26: /Controller/UART_RX -> VDD_3V3
- U1 pad 29: /Controller/M4_I_DCB -> Net-(U1B-ADCINC4_CMPIN5P)
- U1 pad 3: /Controller/M2_I_DCB -> VDD_3V3
- U1 pad 30: unconnected-(U1-ADCA_CH7C-Pad30) -> Net-(U1B-ADCINC3_CMPIN6N)
- U1 pad 31: +3.3VA -> Net-(U1B-ADCINC2_CMPIN6P)
- U1 pad 32: +3.3VA -> GNDD
- U1 pad 35: unconnected-(U1-ADC0_SE0/ADC0_DP0-Pad35) -> Net-(U1B-VREFHIC)
- U1 pad 36: unconnected-(U1-ADC0_SE8/ADC0_DM0-Pad36) -> VDDA_3V3
- U1 pad 37: /Controller/M3_BEMF_B -> Net-(U1B-VREFHIA)
- U1 pad 38: /Controller/M3_BEMF_C -> Net-(U1B-ADCINA5_CMPIN2N)
- U1 pad 39: /Controller/DRV_OC_COM -> Net-(U1B-ADCINA4_CMPIN2P)
- U1 pad 4: /Controller/M3_I_DCB -> /Controller/EPWM7A
- U1 pad 40: unconnected-(U1-PTE13-Pad40) -> Net-(U1B-ADCINA3_CMPIN1N)
- U1 pad 41: unconnected-(U1-FTM2_QD_PHA-Pad41) -> Net-(U1B-ADCINA2_CMPIN1P)
- U1 pad 42: unconnected-(U1-FTM2_QD_PHB-Pad42) -> Net-(U1B-ADCINA1_DACOUTB)
- U1 pad 43: +3.3V -> Net-(U1B-ADCINA0_DACOUTA)
- U1 pad 44: GNDD -> Net-(U1B-ADCIN14_CMPIN4P)
- U1 pad 45: /Controller/M4_BEMF_B -> Net-(U1B-ADCIN15_CMPIN4N)
- U1 pad 46: /Controller/M4_BEMF_C -> Net-(U1B-ADCINB0_VDAC)
- U1 pad 47: /Controller/DRV_RESET -> Net-(U1B-ADCINB1_DACOUTC)
- U1 pad 48: unconnected-(U1-CAN2_TX-Pad48) -> Net-(U1B-ADCINB2_CMPIN3P)
- U1 pad 49: unconnected-(U1-CAN2_RX-Pad49) -> Net-(U1B-ADCINB3_CMPIN3N)
- U1 pad 5: +3.3V -> /Controller/EPWM7B
- U1 pad 50: /Controller/SWDCLK -> GNDD
- U1 pad 51: /Controller/M1_DRV_OC -> GNDD
- U1 pad 52: /Controller/SWO -> GNDD
- U1 pad 53: /Controller/SWDIO -> Net-(U1B-VREFHIB)
- U1 pad 54: /Controller/nmi -> VDDA_3V3
- U1 pad 55: /Controller/M2_DRV_OC -> Net-(U1B-VREFHID)
- U1 pad 56: +3.3V -> Net-(U1B-ADCIND0_CMPIN7P)
- U1 pad 57: GNDD -> Net-(U1B-ADCIND1_CMPIN7N)
- U1 pad 58: unconnected-(U1-PTA6-Pad58) -> Net-(U1B-ADCIND2_CMPIN8P)
- U1 pad 59: unconnected-(U1-PTA7-Pad59) -> Net-(U1B-ADCIND3_CMPIN8N)
- U1 pad 6: GNDD -> /Controller/EPWM8A
- U1 pad 60: unconnected-(U1-PTA8-Pad60) -> Net-(U1B-ADCIND4)
- U1 pad 61: unconnected-(U1-PTA9-Pad61) -> VDD_1V2
- U1 pad 62: unconnected-(U1-PTA10-Pad62) -> VDD_3V3
- U1 pad 63: unconnected-(U1-PTA11-Pad63) -> /Controller/EPWM16A
- U1 pad 66: unconnected-(U1-PTA14-Pad66) -> /Controller/EPWM16B
- U1 pad 68: /Controller/MISO_3V3 -> VDD_3V3
- U1 pad 7: /Controller/M3_DRV_INT -> /Controller/EPWM8B
- U1 pad 70: +3.3V -> unconnected-(U1C-GPIO34-Pad70)
- U1 pad 71: GNDD -> unconnected-(U1C-GPIO35-Pad71)
- U1 pad 72: /Controller/EXTAL_J -> unconnected-(U1E-VDD3VFL-Pad72)
- U1 pad 73: /Controller/XTAL_J -> unconnected-(U1A-FLT1-Pad73)
- U1 pad 74: /Controller/RESET_MCU -> unconnected-(U1A-FLT2-Pad74)
- U1 pad 75: unconnected-(U1-PTA24-Pad75) -> VDD_3V3
- U1 pad 76: unconnected-(U1-PTA25-Pad76) -> VDD_1V2
- U1 pad 77: unconnected-(U1-PTA26-Pad77) -> /controllerConfig/MCU_TDI
- U1 pad 78: unconnected-(U1-PTA27-Pad78) -> Net-(U1A-TDO)
- U1 pad 79: unconnected-(U1-PTA28-Pad79) -> /controllerConfig/MCU_TRSTn
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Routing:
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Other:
- board size 184 x 184 mm -> 100 x 100 mm
